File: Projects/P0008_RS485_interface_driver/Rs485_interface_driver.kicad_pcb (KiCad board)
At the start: 2 copper layers, 36.8 x 22.9 mm, 25 parts, among them J1 22-05-7045, J2 22-05-7035, J3 10118193-0001LF, P1 CONN_01X06, Q1 BSS138, Q2 BSS138, Q3 BSS138, U1 SN65176BDR, U2 FT231XS, U3 TC7W241FUTE12LF

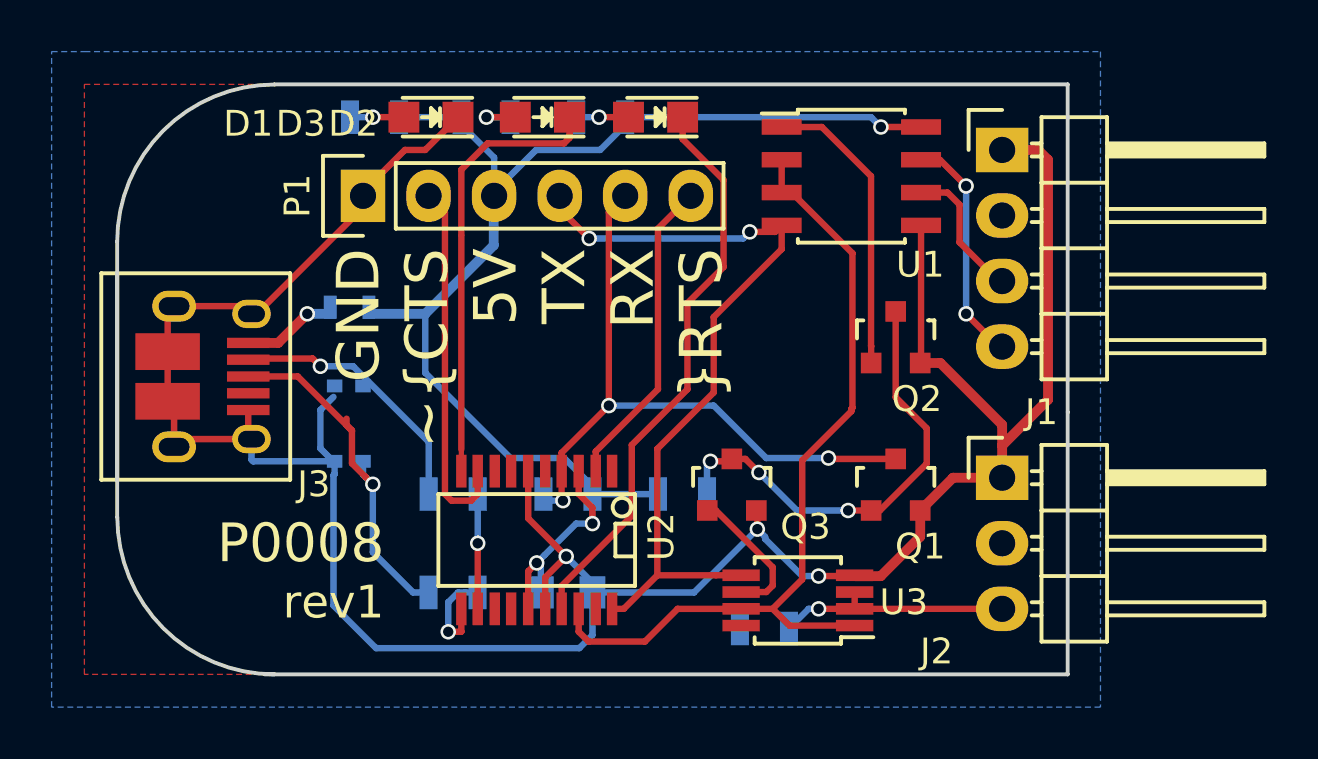
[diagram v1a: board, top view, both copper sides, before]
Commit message: revised P0008, added gerbers
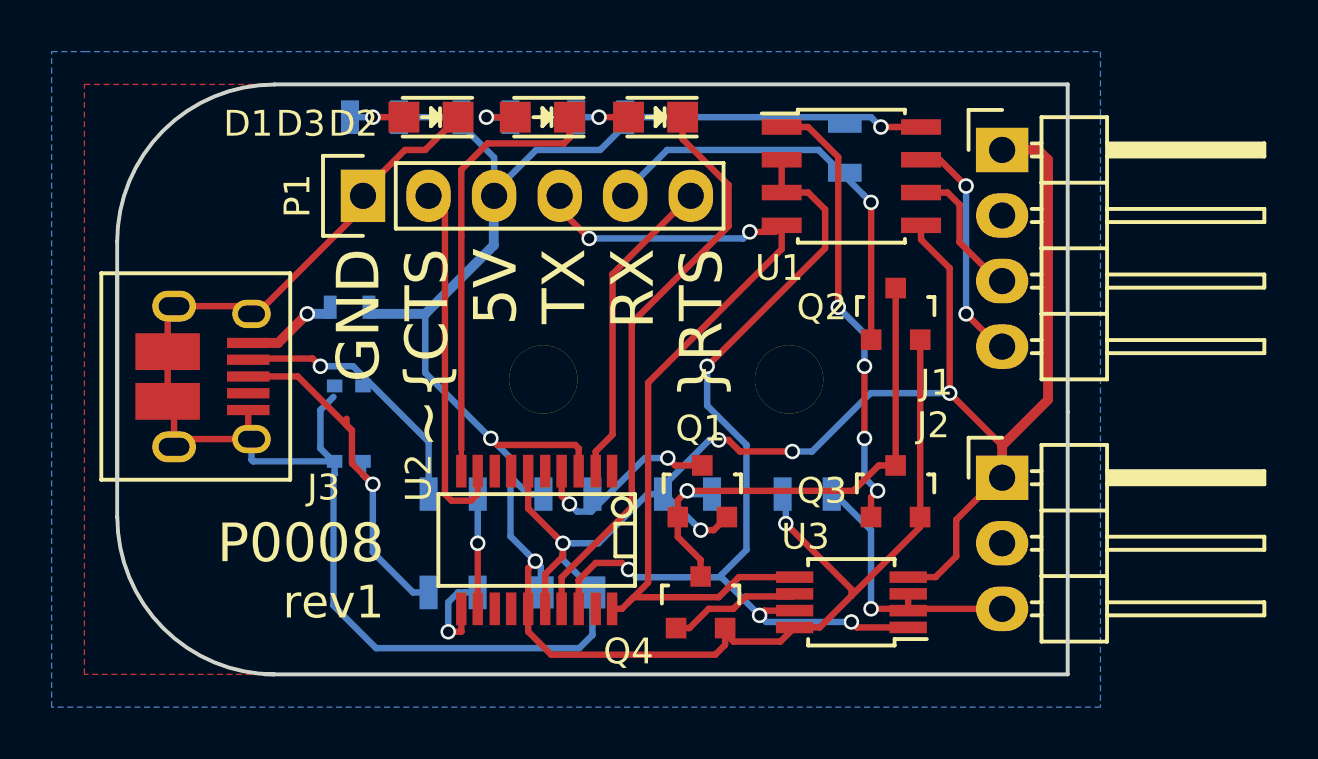
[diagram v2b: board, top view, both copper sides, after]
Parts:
- added Q4: BSS84, TO_SOT_Packages_SMD:SOT-23, F.Cu at (178.8, 100.1)
- added R9: 1k, Resistors_SMD:R_0805, B.Cu at (184.4, 82.5)
- added REF**: modular8_mounting_hole, open_robotics:modular8_mounting_hole, F.Cu at (182.2, 91.4)
- added REF**: modular8_mounting_hole, open_robotics:modular8_mounting_hole, F.Cu at (172.7, 91.4)
- Q2, Q3: value BSS138 -> BSS84
- moved Q1 7.50 mm to (178.9, 95.8)
- moved Q3 6.35 mm to (186.4, 95.8)
- moved R5 5.46 mm to (182.9, 95.9)
- moved U3 2.07 mm to (184.7, 100.1)
- moved Q2 0.90 mm to (186.4, 88.9)
- moved R2 0.19 mm to (178.3, 95.9), turned to 180 degrees
- turned R1 to 0 degrees
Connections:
- P1 pad 5: /RX -> /RX_HEADER
- Q2 pad 1: Net-(Q2-Pad1) -> /RX_HEADER
- Q2 pad 2: GND -> /VCC
- Q3 pad 2: GND -> /VCC
- R2 pad 1: /VCC -> Net-(Q1-Pad1)
- R2 pad 2: Net-(Q1-Pad1) -> GND
- U1 pad 1: Net-(Q2-Pad1) -> Net-(Q3-Pad1)
- U3 pad 6: Net-(Q3-Pad1) -> Net-(Q4-Pad1)
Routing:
- net /VCC: track 54.9 -> 85.2 mm, vias 3 -> 4
- net /RX: track 25.7 -> 7.95 mm, vias 3 -> 2
- net /RX_HEADER: track 0.00 -> 16.5 mm, vias 0 -> 1
- net Net-(Q3-Pad1): track 5.48 -> 17.4 mm, vias 0 -> 4
- net Net-(Q2-Pad1): track 11.5 -> 0.00 mm
- net GND: track 103.8 -> 110.4 mm, vias 3 -> 5
- net Net-(Q4-Pad1): track 0.00 -> 5.14 mm
- net /TXDEN: track 32.5 -> 37.4 mm, vias 0 -> 4
- net /TX: track 30.9 -> 34.4 mm
- net Net-(Q1-Pad1): track 17.7 -> 20.2 mm, vias 3 -> 1
- net /TTL_BUS: track 9.23 -> 11.0 mm
